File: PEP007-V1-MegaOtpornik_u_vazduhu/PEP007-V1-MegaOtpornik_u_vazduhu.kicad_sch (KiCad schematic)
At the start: 8 parts, among them J2 Klema

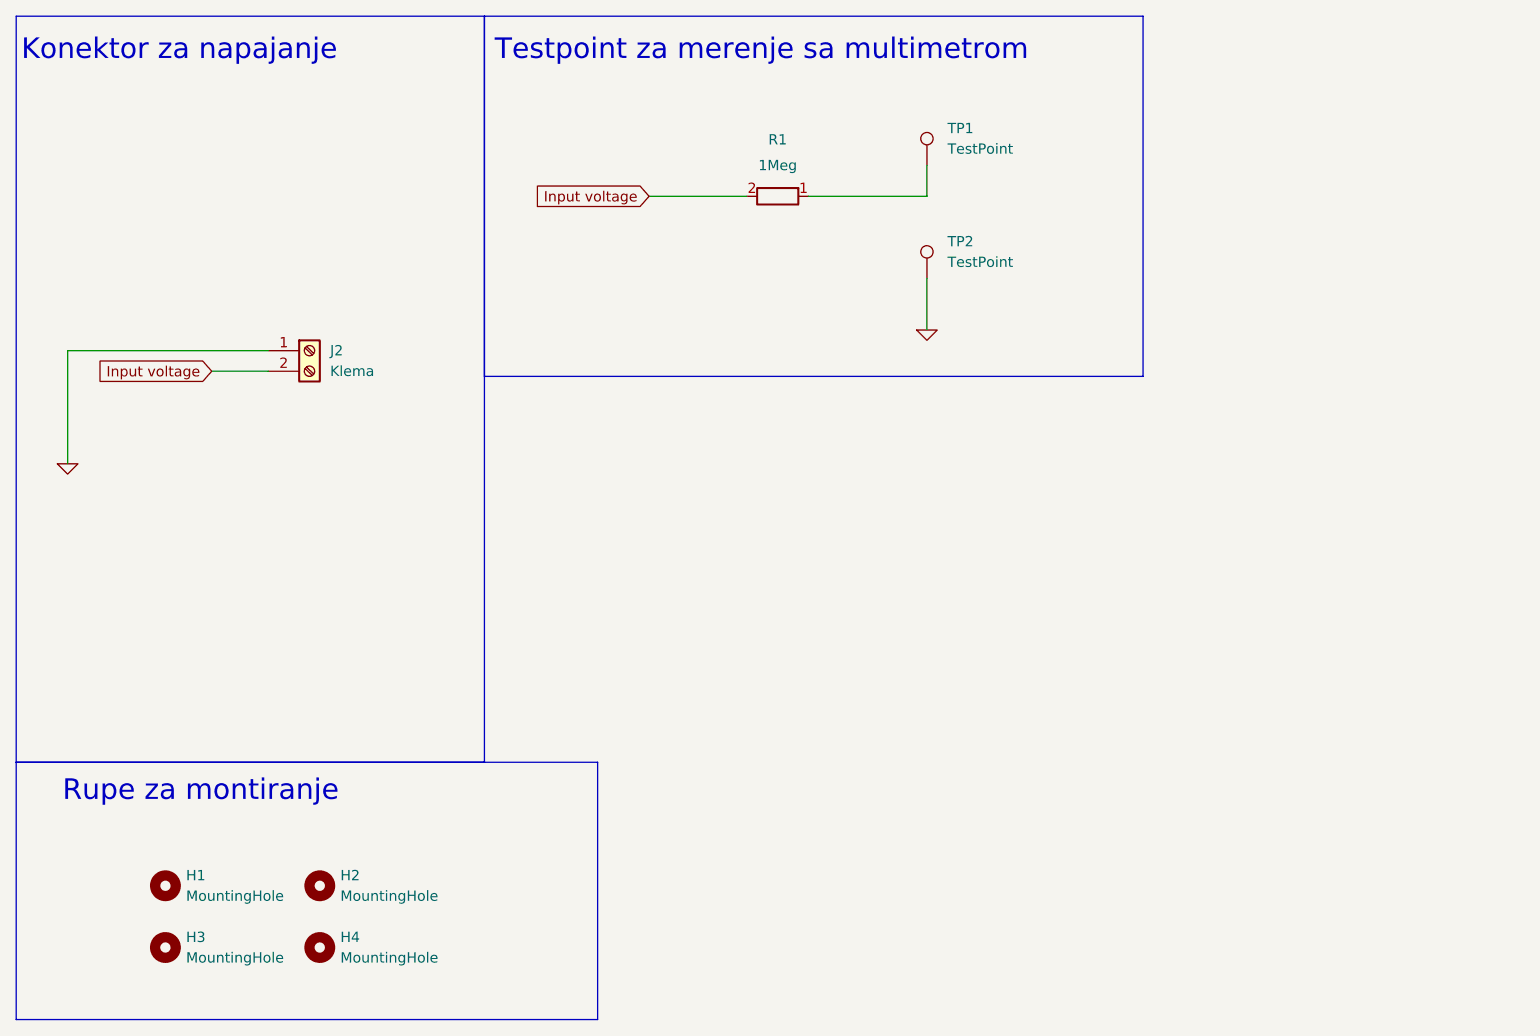
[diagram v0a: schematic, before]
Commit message: PEP007 final update, ready for production.
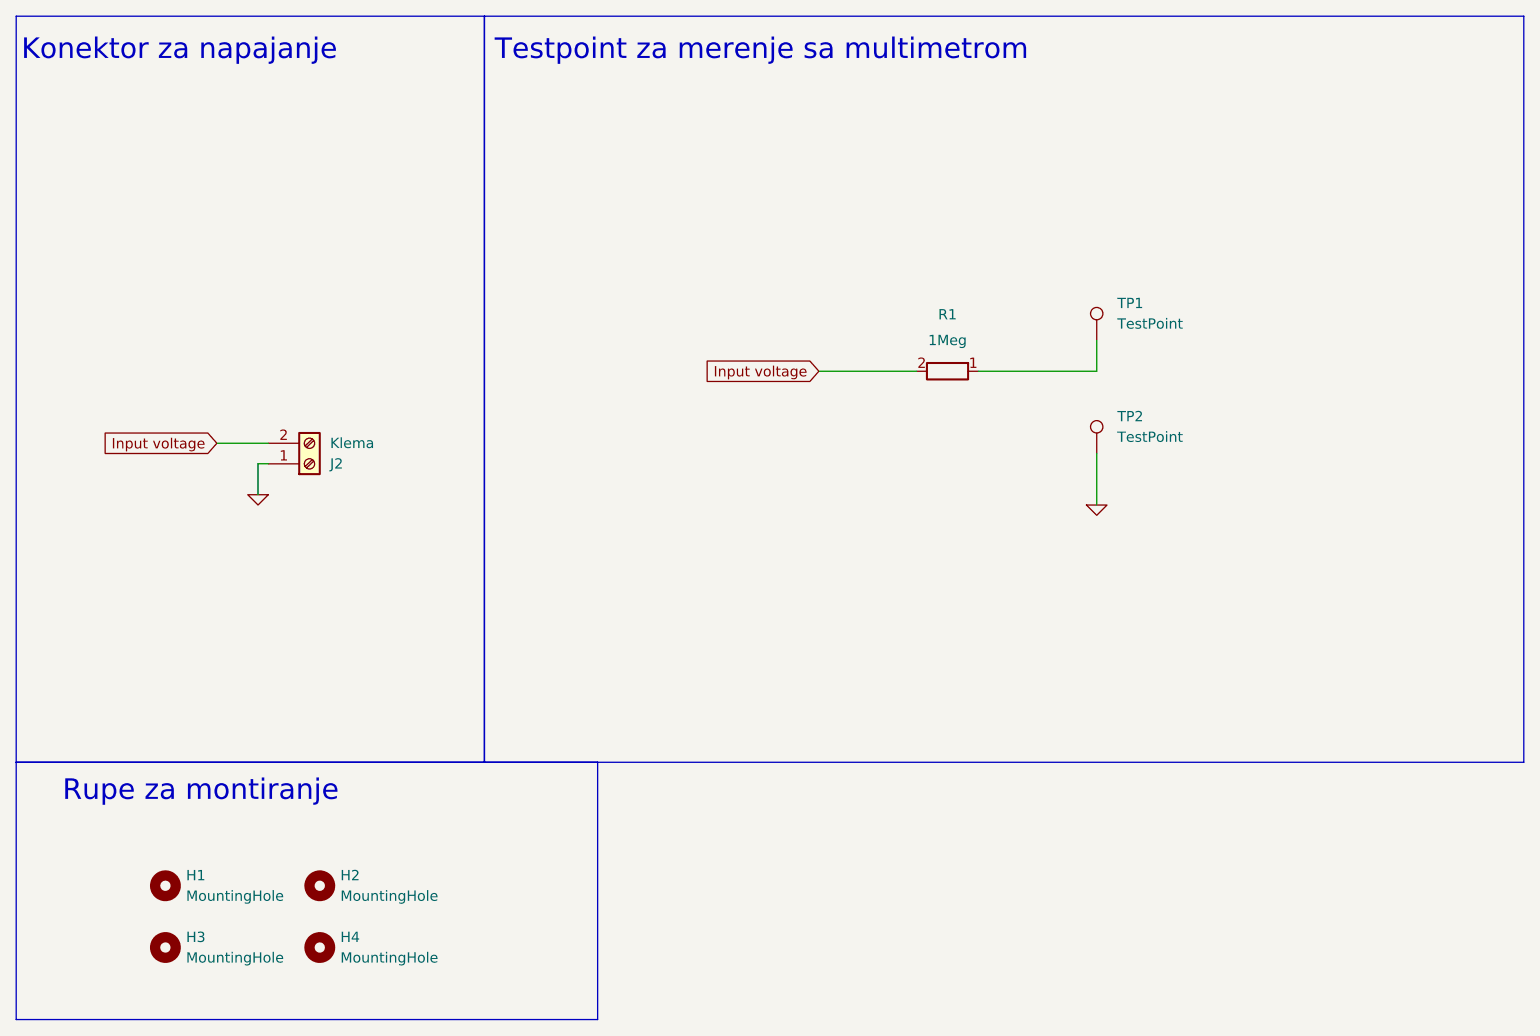
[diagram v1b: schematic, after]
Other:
- moved on the sheet: J2, R1, TP1, TP2
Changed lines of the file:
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@@
 	(wire
 		(pts
-			(xy 124.46 34.29) (xy 109.855 34.29)
+			(xy 145.415 55.88) (xy 130.81 55.88)
 		)
 		(stroke
@@
 	(wire
 		(pts
-			(xy 18.415 53.34) (xy 18.415 67.31)
+			(xy 41.91 67.31) (xy 41.91 71.12)
 		)
 		(stroke
@@
 	(wire
 		(pts
-			(xy 90.17 34.29) (xy 102.235 34.29)
+			(xy 111.125 55.88) (xy 123.19 55.88)
 		)
 		(stroke
@@
 	(wire
 		(pts
-			(xy 36.195 55.88) (xy 43.18 55.88)
+			(xy 36.83 64.77) (xy 43.18 64.77)
 		)
 		(stroke
@@
 	(wire
 		(pts
-			(xy 124.46 44.45) (xy 124.46 50.8)
+			(xy 145.415 66.04) (xy 145.415 72.39)
 		)
 		(stroke
@@
 	(wire
 		(pts
-			(xy 18.415 53.34) (xy 43.18 53.34)
+			(xy 41.91 67.31) (xy 43.18 67.31)
 		)
 		(stroke
@@
 	(wire
 		(pts
-			(xy 124.46 30.48) (xy 124.46 34.29)
+			(xy 145.415 52.07) (xy 145.415 55.88)
 		)
 		(stroke
@@
 	(rectangle
 		(start 69.85 12.065)
-		(end 151.13 56.515)
+		(end 198.12 104.14)
 		(stroke
 			(width 0)
@@
 	(global_label "Input voltage"
 		(shape input)
-		(at 36.195 55.88 180)
+		(at 36.83 64.77 180)
 		(fields_autoplaced yes)
 		(effects
@@
 		)
 		(property "Intersheetrefs" "${INTERSHEET_REFS}"
-			(at 20.5706 55.88 0)
+			(at 21.2056 64.77 0)
 			(effects
 				(font
@@
 	(global_label "Input voltage"
 		(shape input)
-		(at 90.17 34.29 180)
+		(at 111.125 55.88 180)
 		(fields_autoplaced yes)
 		(effects
@@
 		)
 		(property "Intersheetrefs" "${INTERSHEET_REFS}"
-			(at 74.5456 34.29 0)
+			(at 95.5006 55.88 0)
 			(effects
 				(font
@@
 	(symbol
 		(lib_id "Simulation_SPICE:0")
-		(at 18.415 67.31 0)
+		(at 41.91 71.12 0)
+		(mirror y)
 		(unit 1)
 		(exclude_from_sim no)
@@
 		(fields_autoplaced yes)
 		(property "Reference" "#GND05"
-			(at 18.415 69.85 0)
+			(at 41.91 73.66 0)
 			(effects
 				(font
@@
 		)
 		(property "Value" "0"
-			(at 18.415 64.77 0)
+			(at 41.91 68.58 0)
 			(effects
 				(font
@@
 		)
 		(property "Footprint" ""
-			(at 18.415 67.31 0)
+			(at 41.91 71.12 0)
 			(effects
 				(font
@@
 		)
 		(property "Datasheet" "~"
-			(at 18.415 67.31 0)
+			(at 41.91 71.12 0)
 			(effects
 				(font
@@
 		)
 		(property "Description" ""
-			(at 18.415 67.31 0)
+			(at 41.91 71.12 0)
 			(effects
 				(font
@@
 	(symbol
 		(lib_id "Connector:TestPoint")
-		(at 124.46 44.45 0)
+		(at 145.415 66.04 0)
 		(unit 1)
 		(exclude_from_sim no)
@@
 		(fields_autoplaced yes)
 		(property "Reference" "TP2"
-			(at 127 39.8779 0)
+			(at 147.955 61.4679 0)
 			(effects
 				(font
@@
 		)
 		(property "Value" "TestPoint"
-			(at 127 42.4179 0)
+			(at 147.955 64.0079 0)
 			(effects
 				(font
@@
 		)
 		(property "Footprint" ""
-			(at 129.54 44.45 0)
+			(at 150.495 66.04 0)
 			(effects
 				(font
@@
 		)
 		(property "Datasheet" "~"
-			(at 129.54 44.45 0)
+			(at 150.495 66.04 0)
 			(effects
 				(font
@@
 		)
 		(property "Description" "test point"
-			(at 124.46 44.45 0)
+			(at 145.415 66.04 0)
 			(effects
 				(font
@@
 	(symbol
 		(lib_id "PEP_library:Klema")
-		(at 48.26 53.34 0)
+		(at 48.26 67.31 0)
+		(mirror x)
 		(unit 1)
 		(exclude_from_sim no)
@@
 		(fields_autoplaced yes)
 		(property "Reference" "J2"
-			(at 50.8 53.3399 0)
+			(at 50.8 67.3101 0)
 			(effects
 				(font
@@
 		)
 		(property "Value" "Klema"
-			(at 50.8 55.8799 0)
+			(at 50.8 64.7701 0)
 			(effects
 				(font
@@
 		)
 		(property "Footprint" "PEP_library:TerminalBlock_Phoenix_MKDS-1,5-2-5.08_1x02_P5.08mm_Horizontal"
-			(at 48.26 53.34 0)
+			(at 48.26 67.31 0)
 			(effects
 				(font
@@
 		)
 		(property "Datasheet" "~"
-			(at 48.26 53.34 0)
+			(at 48.26 67.31 0)
 			(effects
 				(font
@@
 		)
 		(property "Description" "Generic screw terminal, single row, 01x02, script generated (kicad-library-utils/schlib/autogen/connector/)"
-			(at 48.26 53.34 0)
+			(at 48.26 67.31 0)
 			(effects
 				(font
@@
 		)
 		(property "LCSC" "C474952"
-			(at 48.26 53.34 0)
+			(at 48.26 67.31 0)
 			(effects
 				(font
@@
 	(symbol
 		(lib_id "Connector:TestPoint")
-		(at 124.46 30.48 0)
+		(at 145.415 52.07 0)
 		(unit 1)
 		(exclude_from_sim no)
@@
 		(fields_autoplaced yes)
 		(property "Reference" "TP1"
-			(at 127 25.9079 0)
+			(at 147.955 47.4979 0)
 			(effects
 				(font
@@
 		)
 		(property "Value" "TestPoint"
-			(at 127 28.4479 0)
+			(at 147.955 50.0379 0)
 			(effects
 				(font
@@
 		)
 		(property "Footprint" ""
-			(at 129.54 30.48 0)
+			(at 150.495 52.07 0)
 			(effects
 				(font
@@
 		)
 		(property "Datasheet" "~"
-			(at 129.54 30.48 0)
+			(at 150.495 52.07 0)
 			(effects
 				(font
@@
 		)
 		(property "Description" "test point"
-			(at 124.46 30.48 0)
+			(at 145.415 52.07 0)
 			(effects
 				(font
@@
 	(symbol
 		(lib_id "Simulation_SPICE:0")
-		(at 124.46 50.8 0)
+		(at 145.415 72.39 0)
 		(unit 1)
 		(exclude_from_sim no)
@@
 		(fields_autoplaced yes)
 		(property "Reference" "#GND01"
-			(at 124.46 53.34 0)
+			(at 145.415 74.93 0)
 			(effects
 				(font
@@
 		)
 		(property "Value" "0"
-			(at 124.46 48.26 0)
+			(at 145.415 69.85 0)
 			(effects
 				(font
@@
 		)
 		(property "Footprint" ""
-			(at 124.46 50.8 0)
+			(at 145.415 72.39 0)
 			(effects
 				(font
@@
 		)
 		(property "Datasheet" "~"
-			(at 124.46 50.8 0)
+			(at 145.415 72.39 0)
 			(effects
 				(font
@@
 		)
 		(property "Description" ""
-			(at 124.46 50.8 0)
+			(at 145.415 72.39 0)
 			(effects
 				(font
@@
 	(symbol
 		(lib_id "PEP_library:R_THT")
-		(at 106.045 34.29 270)
+		(at 127 55.88 270)
 		(unit 1)
 		(exclude_from_sim no)
@@
 		(dnp no)
 		(property "Reference" "R1"
-			(at 106.045 27.305 90)
+			(at 127 48.895 90)
 			(effects
 				(font
@@
 		)
 		(property "Value" "1Meg"
-			(at 106.045 30.48 90)
+			(at 127 52.07 90)
 			(effects
 				(font
@@
 		)
 		(property "Footprint" "PEP_library:R_Axial_DIN0207_L6.3mm_D2.5mm_P15.24mm_Horizontal"
-			(at 102.743 34.29 0)
+			(at 123.698 55.88 0)
 			(effects
 				(font
@@
 		)
 		(property "Datasheet" ""
-			(at 106.045 34.29 0)
+			(at 127 55.88 0)
 			(effects
 				(font
@@
 		)
 		(property "Description" ""
-			(at 106.045 34.29 0)
+			(at 127 55.88 0)
 			(effects
 				(font
@@
 		)
 		(property "Size" ""
-			(at 106.045 31.115 90)
+			(at 127 52.705 90)
 			(effects
 				(font
@@
 		)
 		(property "Power rating" ""
-			(at 106.045 34.29 0)
+			(at 127 55.88 0)
 			(effects
 				(font
@@
 		)
 		(property "LCSC" "C2903250"
-			(at 106.045 34.29 90)
-			(effects
-				(font
+			(at 127 55.88 90)
+			(effects
+				(font
